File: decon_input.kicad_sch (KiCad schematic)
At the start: 35 parts, among them J21 Conn_01x02, U1 LTV-817S, U2 LTV-817S, U22 LTV-817S, U23 LTV-817S, U24 LTV-817S, U25 LTV-817S, U4 LTV-817S, U5 LTV-817S

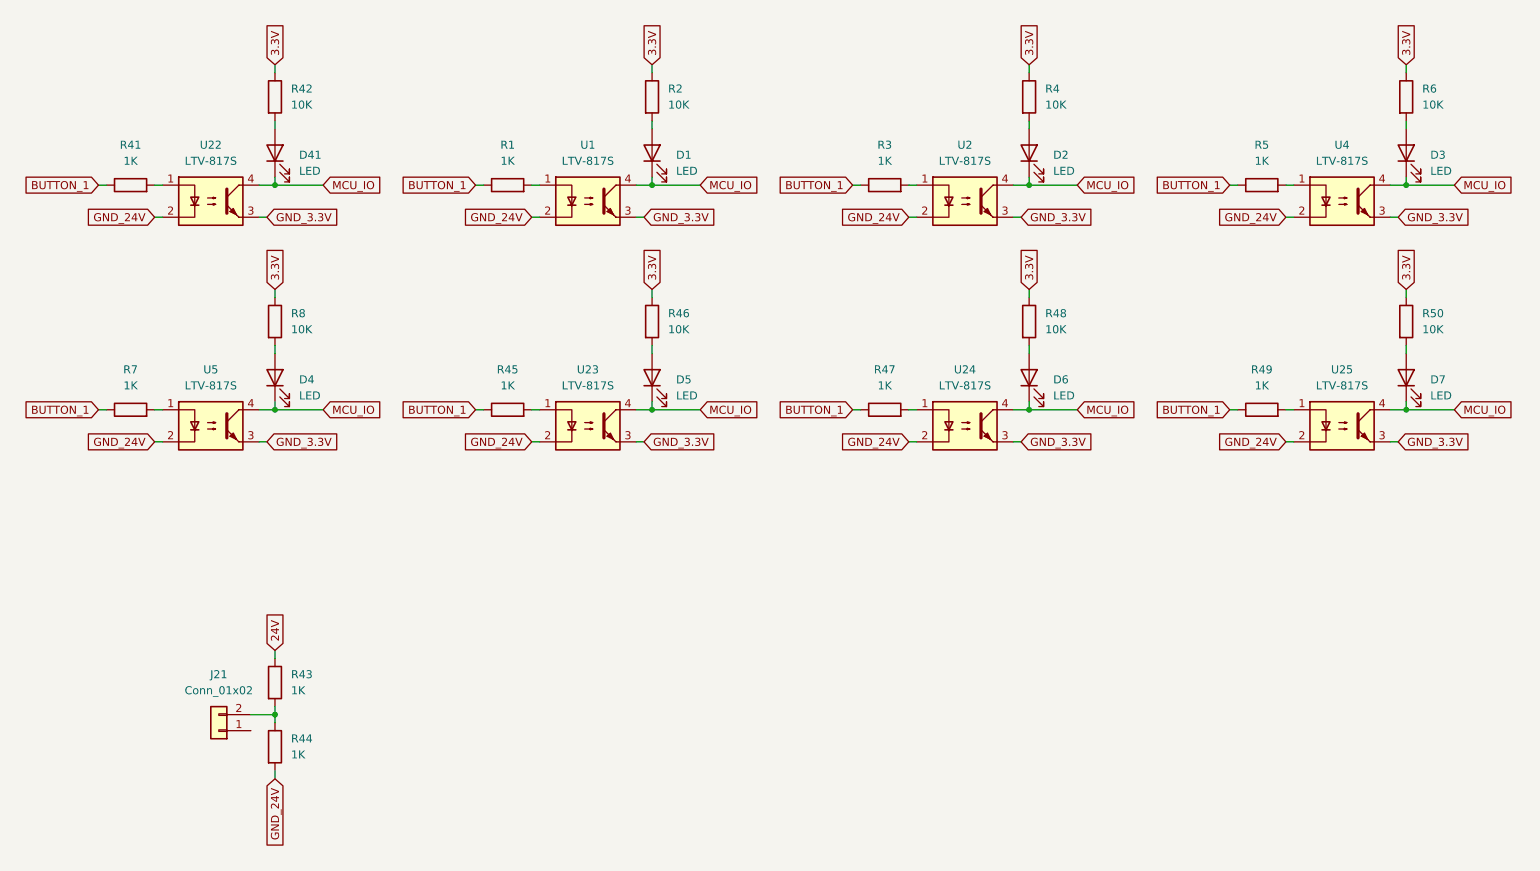
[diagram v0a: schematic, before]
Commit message: modified:   DECON_Ctrl_Panel.kicad_pcb 	modified:   DECON_Ctrl_Panel.kicad_prl 	new file:   MCU_pins.xlsx 	new file:   Son_KiCad_lib/Son_KiCad_lib.bak 	new file:   Son_KiCad_lib/Son_KiCad_lib.kicad_sym 	new file:   Son_KiCad_lib/Son_KiCad_lib.pretty/URB2405YMD-10WR3.kicad_mod 	modified:   decon_input.kicad_sch 	modified:   decon_mcu.kicad_sch 	modified:   decon_output.kicad_sch 	modified:   decon_power.kicad_sch 	new file:   fp-lib-table 	new file:   sym-lib-table
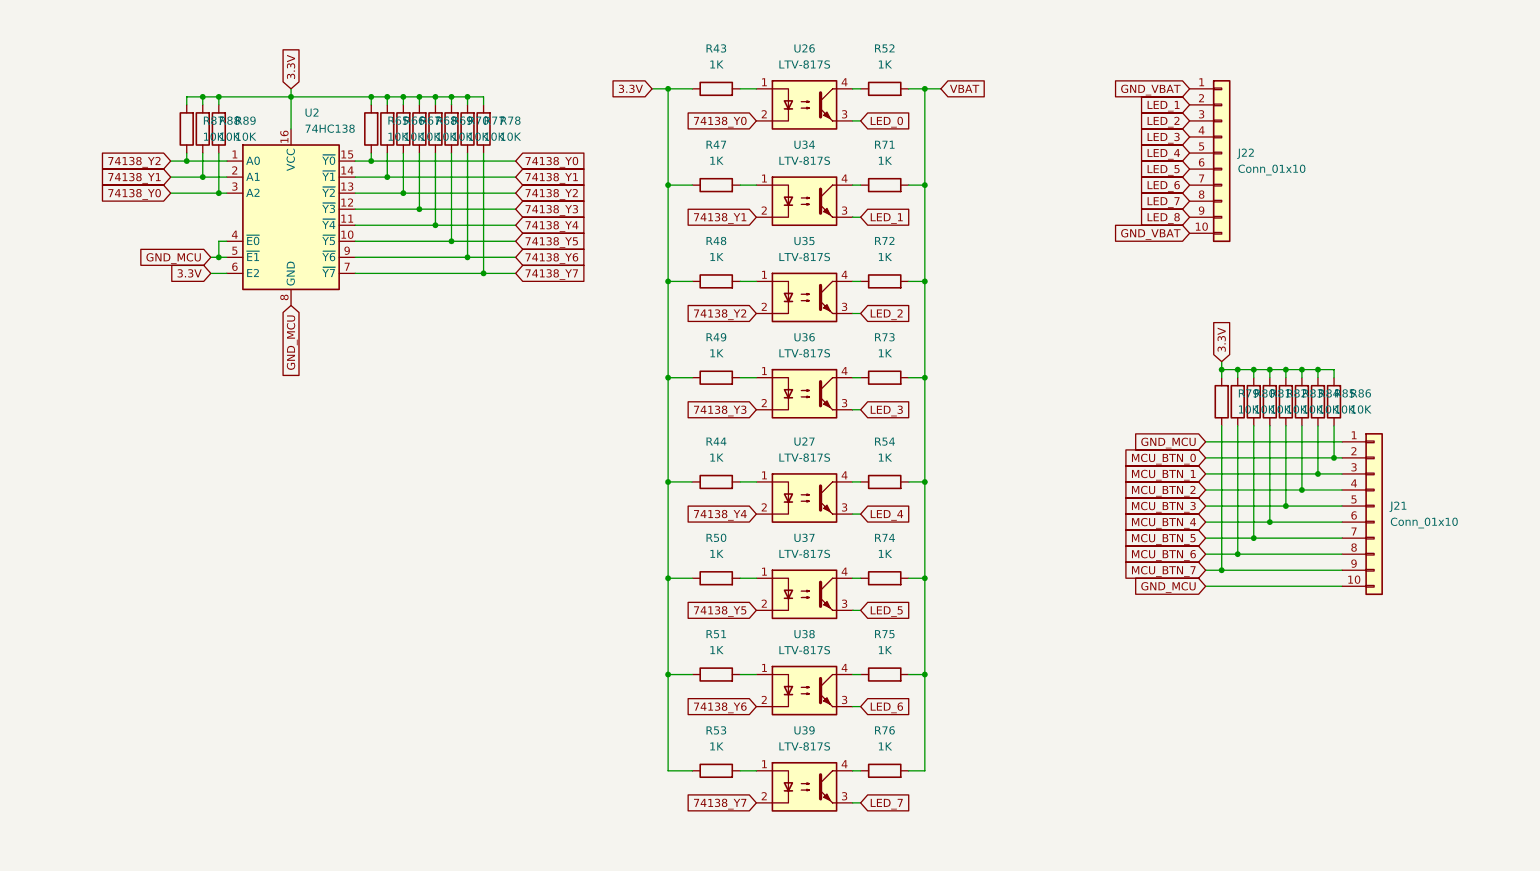
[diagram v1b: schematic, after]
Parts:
- removed D1, D2, D3, D4, D41, D5, D6, D7: LED, LED_SMD:LED_0805_2012Metric, symbol Device:LED
- removed J21: Conn_01x02, TerminalBlock_Phoenix:TerminalBlock_Phoenix_MKDS-1-2-3.81_1x02_P3.81mm_Horizontal, symbol Connector_Generic:Conn_01x02
- removed R1, R3, R41, R45, R5, R7: 1K, Resistor_SMD:R_0805_2012Metric, symbol Device:R
- removed R2, R4, R42, R46, R6, R8: 10K, Resistor_SMD:R_0805_2012Metric, symbol Device:R
- removed U1, U2, U22, U23, U24, U25, U4, U5: LTV-817S, Package_DIP:SMDIP-4_W9.53mm, symbol Isolator:LTV-817S
- added J21, J22: Conn_01x10, Connector_Phoenix_MC:PhoenixContact_MC_1,5_10-G-3.81_1x10_P3.81mm_Horizontal, symbol Connector_Generic:Conn_01x10
- added R51, R52, R53, R54, R71, R72, R73, R74, R75, R76: 1K, Resistor_SMD:R_0805_2012Metric, symbol Device:R
- added R65, R66, R67, R68, R69, R70, R77, R78, R79, R80, R81, R82, R83, R84, R85, R86, R87, R88, R89: 10K, Resistor_SMD:R_0805_2012Metric, symbol Device:R
- added U2: 74HC138, Package_SO:SOIC-16_3.9x9.9mm_P1.27mm, symbol 74xx:74HC138
- added U26, U27, U34, U35, U36, U37, U38, U39: LTV-817S, Package_DIP:SMDIP-4_W9.53mm, symbol Isolator:LTV-817S
- R48, R50: value 10K -> 1K
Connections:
- net 24V is gone; now on net 3.3V: R43.1
- net BUTTON_1 is gone; now on net 3.3V: R47.1, R49.1
- net 3.3V: now also R44.1, R51.1, R53.1, R65.2, R66.2, R67.2, R68.2, R69.2, R70.2, R77.2, R78.2, R79.2, R80.2, R81.2, R82.2, R83.2, R84.2, R85.2, R86.2, R87.2, R88.2, R89.2, U2.16 (VCC), U2.6 (E2)
- net at R47.2: now also U34.1
- net at R49.2: now also U36.1
- net at R48.2: now also U35.1
- net at R43.2: now also U26.1; no longer R44.1
- net at R50.2: now also U37.1
- net GND_24V: no longer names the net of R44.2
- net GND_24V: now also U27.1
- new net: R52.1, U26.4
- new net: R71.1, U34.4
- new net: R51.2, U38.1
- new net: R53.2, U39.1
- new net: R76.1, U39.4
- new net: R73.1, U36.4
- new net: R54.1, U27.4
- new net: R72.1, U35.4
- new net: R74.1, U37.4
- new net: R75.1, U38.4
- new net 74138_Y0: R65.1, R89.1, U2.15 (~{Y0}), U2.3 (A2), U26.2
- new net 74138_Y1: R66.1, R88.1, U2.14 (~{Y1}), U2.2 (A1), U34.2
- new net 74138_Y2: R67.1, R87.1, U2.1 (A0), U2.13 (~{Y2}), U35.2
- new net 74138_Y3: R68.1, U2.12 (~{Y3}), U36.2
- new net 74138_Y4: R69.1, U2.11 (~{Y4}), U27.2
- new net 74138_Y5: R70.1, U2.10 (~{Y5}), U37.2
- new net 74138_Y6: R77.1, U2.9 (~{Y6}), U38.2
- new net 74138_Y7: R78.1, U2.7 (~{Y7}), U39.2
- new net GND_MCU: J21.1 (Pin_1), J21.10 (Pin_10), U2.4 (~{E0}), U2.5 (~{E1}), U2.8 (GND)
- new net GND_VBAT: J22.1 (Pin_1), J22.10 (Pin_10)
- new net LED_0: U26.3
- new net LED_1: J22.2 (Pin_2), U34.3
- new net LED_2: J22.3 (Pin_3), U35.3
- new net LED_3: J22.4 (Pin_4), U36.3
- new net LED_4: J22.5 (Pin_5), U27.3
- new net LED_5: J22.6 (Pin_6), U37.3
- new net LED_6: J22.7 (Pin_7), U38.3
- new net LED_7: J22.8 (Pin_8), U39.3
- new net LED_8: J22.9 (Pin_9)
- new net MCU_BTN_0: J21.2 (Pin_2), R86.1
- new net MCU_BTN_1: J21.3 (Pin_3), R85.1
- new net MCU_BTN_2: J21.4 (Pin_4), R84.1
- new net MCU_BTN_3: J21.5 (Pin_5), R83.1
- new net MCU_BTN_4: J21.6 (Pin_6), R82.1
- new net MCU_BTN_5: J21.7 (Pin_7), R81.1
- new net MCU_BTN_6: J21.8 (Pin_8), R80.1
- new net MCU_BTN_7: J21.9 (Pin_9), R79.1
- new net VBAT: R52.2, R54.2, R71.2, R72.2, R73.2, R74.2, R75.2, R76.2
